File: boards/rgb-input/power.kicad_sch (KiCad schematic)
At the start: 18 parts, among them J1 Barrel_Jack, U3 XL1509-5.0

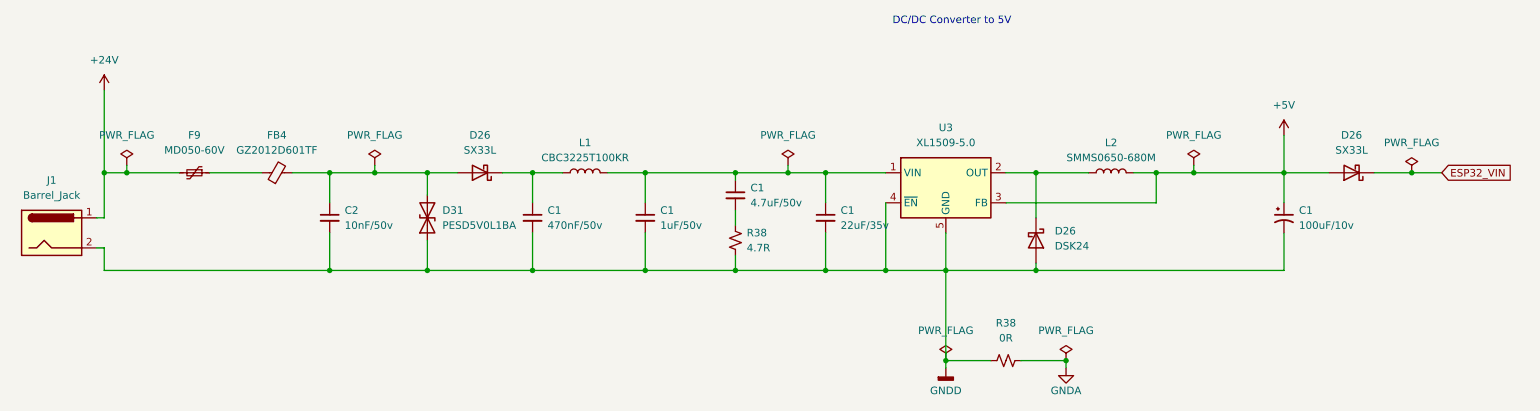
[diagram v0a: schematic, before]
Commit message: various cleanups and tidying
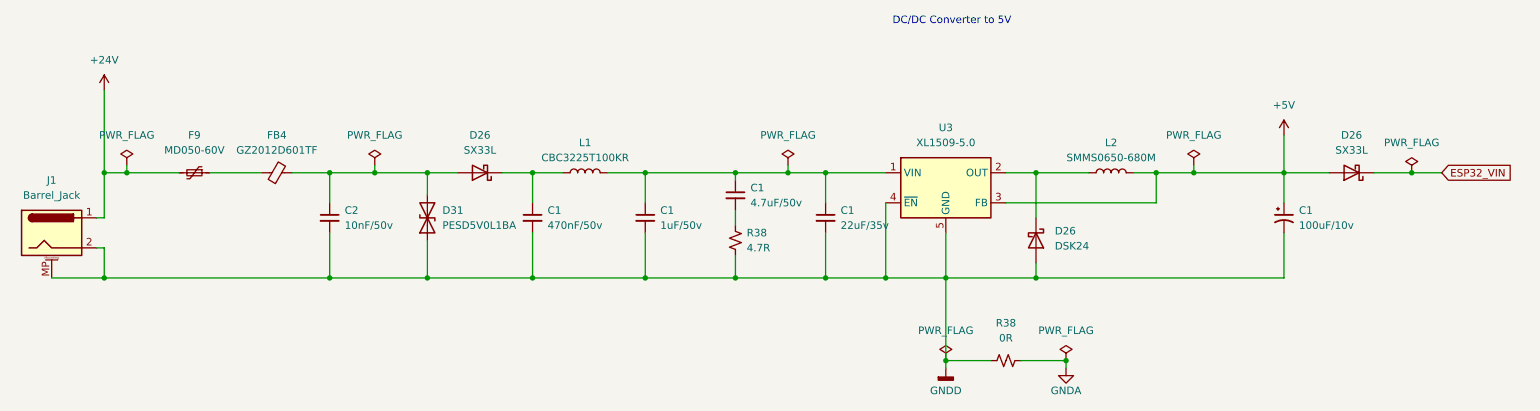
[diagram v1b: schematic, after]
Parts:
- J1: symbol Connector:Barrel_Jack -> Connector:Barrel_Jack_MountingPin
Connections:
- net GNDD: now also J1.MP (MountPin)
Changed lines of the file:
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@@
   (junction (at 173.99 111.76) (diameter 0) (color 0 0 0 0)
   )
+  (junction (at 31.75 97.79) (diameter 0) (color 0 0 0 0)
+  )
   (junction (at 31.75 80.01) (diameter 0) (color 0 0 0 0)
   )
   (junction (at 69.85 80.01) (diameter 0) (color 0 0 0 0)
   )
-  (junction (at 173.99 96.52) (diameter 0) (color 0 0 0 0)
+  (junction (at 173.99 97.79) (diameter 0) (color 0 0 0 0)
   )
   (junction (at 209.55 80.01) (diameter 0) (color 0 0 0 0)
@@
   (junction (at 231.14 80.01) (diameter 0) (color 0 0 0 0)
   )
-  (junction (at 189.23 96.52) (diameter 0) (color 0 0 0 0)
-  )
-  (junction (at 123.19 96.52) (diameter 0) (color 0 0 0 0)
-  )
-  (junction (at 163.83 96.52) (diameter 0) (color 0 0 0 0)
-  )
-  (junction (at 69.85 96.52) (diameter 0) (color 0 0 0 0)
+  (junction (at 189.23 97.79) (diameter 0) (color 0 0 0 0)
+  )
+  (junction (at 123.19 97.79) (diameter 0) (color 0 0 0 0)
+  )
+  (junction (at 163.83 97.79) (diameter 0) (color 0 0 0 0)
+  )
+  (junction (at 69.85 97.79) (diameter 0) (color 0 0 0 0)
   )
   (junction (at 86.36 80.01) (diameter 0) (color 0 0 0 0)
   )
-  (junction (at 153.67 96.52) (diameter 0) (color 0 0 0 0)
+  (junction (at 153.67 97.79) (diameter 0) (color 0 0 0 0)
   )
   (junction (at 35.56 80.01) (diameter 0) (color 0 0 0 0)
@@
   (junction (at 153.67 80.01) (diameter 0) (color 0 0 0 0)
   )
-  (junction (at 104.14 96.52) (diameter 0) (color 0 0 0 0)
+  (junction (at 104.14 97.79) (diameter 0) (color 0 0 0 0)
   )
   (junction (at 252.73 80.01) (diameter 0) (color 0 0 0 0)
@@
   (junction (at 77.47 80.01) (diameter 0) (color 0 0 0 0)
   )
-  (junction (at 138.43 96.52) (diameter 0) (color 0 0 0 0)
+  (junction (at 138.43 97.79) (diameter 0) (color 0 0 0 0)
   )
   (junction (at 147.32 80.01) (diameter 0) (color 0 0 0 0)
   )
-  (junction (at 86.36 96.52) (diameter 0) (color 0 0 0 0)
-  )
-  (wire (pts (xy 138.43 96.52) (xy 153.67 96.52))
-    (stroke (width 0) (type default))
-  )
-  (wire (pts (xy 138.43 93.98) (xy 138.43 96.52))
+  (junction (at 86.36 97.79) (diameter 0) (color 0 0 0 0)
+  )
+  (wire (pts (xy 138.43 97.79) (xy 153.67 97.79))
+    (stroke (width 0) (type default))
+  )
+  (wire (pts (xy 138.43 93.98) (xy 138.43 97.79))
     (stroke (width 0) (type default))
   )
@@
     (stroke (width 0) (type default))
   )
-  (wire (pts (xy 69.85 90.17) (xy 69.85 96.52))
+  (wire (pts (xy 69.85 90.17) (xy 69.85 97.79))
     (stroke (width 0) (type default))
   )
@@
     (stroke (width 0) (type default))
   )
-  (wire (pts (xy 123.19 96.52) (xy 138.43 96.52))
+  (wire (pts (xy 123.19 97.79) (xy 138.43 97.79))
+    (stroke (width 0) (type default))
+  )
+  (wire (pts (xy 22.86 97.79) (xy 31.75 97.79))
     (stroke (width 0) (type default))
   )
@@
     (stroke (width 0) (type default))
   )
-  (wire (pts (xy 31.75 96.52) (xy 31.75 92.71))
-    (stroke (width 0) (type default))
-  )
-  (wire (pts (xy 173.99 96.52) (xy 189.23 96.52))
+  (wire (pts (xy 31.75 97.79) (xy 31.75 92.71))
+    (stroke (width 0) (type default))
+  )
+  (wire (pts (xy 173.99 97.79) (xy 189.23 97.79))
     (stroke (width 0) (type default))
   )
@@
     (stroke (width 0) (type default))
   )
-  (wire (pts (xy 153.67 96.52) (xy 163.83 96.52))
-    (stroke (width 0) (type default))
-  )
-  (wire (pts (xy 163.83 85.09) (xy 163.83 96.52))
+  (wire (pts (xy 153.67 97.79) (xy 163.83 97.79))
+    (stroke (width 0) (type default))
+  )
+  (wire (pts (xy 163.83 85.09) (xy 163.83 97.79))
     (stroke (width 0) (type default))
   )
@@
     (stroke (width 0) (type default))
   )
-  (wire (pts (xy 153.67 90.17) (xy 153.67 96.52))
+  (wire (pts (xy 153.67 90.17) (xy 153.67 97.79))
     (stroke (width 0) (type default))
   )
@@
     (stroke (width 0) (type default))
   )
-  (wire (pts (xy 163.83 96.52) (xy 173.99 96.52))
-    (stroke (width 0) (type default))
-  )
-  (wire (pts (xy 86.36 91.44) (xy 86.36 96.52))
+  (wire (pts (xy 163.83 97.79) (xy 173.99 97.79))
+    (stroke (width 0) (type default))
+  )
+  (wire (pts (xy 86.36 91.44) (xy 86.36 97.79))
     (stroke (width 0) (type default))
   )
@@
     (stroke (width 0) (type default))
   )
-  (wire (pts (xy 69.85 96.52) (xy 31.75 96.52))
+  (wire (pts (xy 69.85 97.79) (xy 31.75 97.79))
     (stroke (width 0) (type default))
   )
@@
     (stroke (width 0) (type default))
   )
-  (wire (pts (xy 69.85 96.52) (xy 86.36 96.52))
+  (wire (pts (xy 69.85 97.79) (xy 86.36 97.79))
     (stroke (width 0) (type default))
   )
@@
     (stroke (width 0) (type default))
   )
-  (wire (pts (xy 173.99 96.52) (xy 173.99 111.76))
+  (wire (pts (xy 173.99 97.79) (xy 173.99 111.76))
     (stroke (width 0) (type default))
   )
@@
     (stroke (width 0) (type default))
   )
-  (wire (pts (xy 189.23 96.52) (xy 231.14 96.52))
+  (wire (pts (xy 189.23 97.79) (xy 231.14 97.79))
     (stroke (width 0) (type default))
   )
@@
     (stroke (width 0) (type default))
   )
-  (wire (pts (xy 189.23 95.25) (xy 189.23 96.52))
+  (wire (pts (xy 189.23 95.25) (xy 189.23 97.79))
     (stroke (width 0) (type default))
   )
@@
     (stroke (width 0) (type default))
   )
-  (wire (pts (xy 104.14 96.52) (xy 123.19 96.52))
-    (stroke (width 0) (type default))
-  )
-  (wire (pts (xy 123.19 90.17) (xy 123.19 96.52))
+  (wire (pts (xy 104.14 97.79) (xy 123.19 97.79))
+    (stroke (width 0) (type default))
+  )
+  (wire (pts (xy 123.19 90.17) (xy 123.19 97.79))
     (stroke (width 0) (type default))
   )
@@
     (stroke (width 0) (type default))
   )
-  (wire (pts (xy 86.36 96.52) (xy 104.14 96.52))
-    (stroke (width 0) (type default))
-  )
-  (wire (pts (xy 231.14 90.17) (xy 231.14 96.52))
+  (wire (pts (xy 86.36 97.79) (xy 104.14 97.79))
+    (stroke (width 0) (type default))
+  )
+  (wire (pts (xy 231.14 90.17) (xy 231.14 97.79))
     (stroke (width 0) (type default))
   )
@@
     (stroke (width 0) (type default))
   )
-  (wire (pts (xy 104.14 90.17) (xy 104.14 96.52))
+  (wire (pts (xy 104.14 90.17) (xy 104.14 97.79))
     (stroke (width 0) (type default))
   )
@@
     (stroke (width 0) (type default))
   )
-  (wire (pts (xy 173.99 90.17) (xy 173.99 96.52))
+  (wire (pts (xy 173.99 90.17) (xy 173.99 97.79))
     (stroke (width 0) (type default))
   )
@@
     )
   )
-  (symbol (lib_id "Connector:Barrel_Jack") (at 22.86 90.17 0) (unit 1)
+  (symbol (lib_id "Connector:Barrel_Jack_MountingPin") (at 22.86 90.17 0) (unit 1)
     (in_bom yes) (on_board yes) (dnp no) (fields_autoplaced)
     (property "Reference" "J1" (at 22.86 81.28 0)
@@
     (pin "1")
     (pin "2")
-    (instances
-      (project "rgb-input"
+    (pin "MP")
+    (instances
+      (project "rgb-input"
